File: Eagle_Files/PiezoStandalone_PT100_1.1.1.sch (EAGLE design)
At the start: 67 parts, among them J1 CON-MOLEX-4P-1.25MM048, U1 ATMEGA48PA-MMHR28M1-L, U2 L78L05ACU, U3 LM2902QT

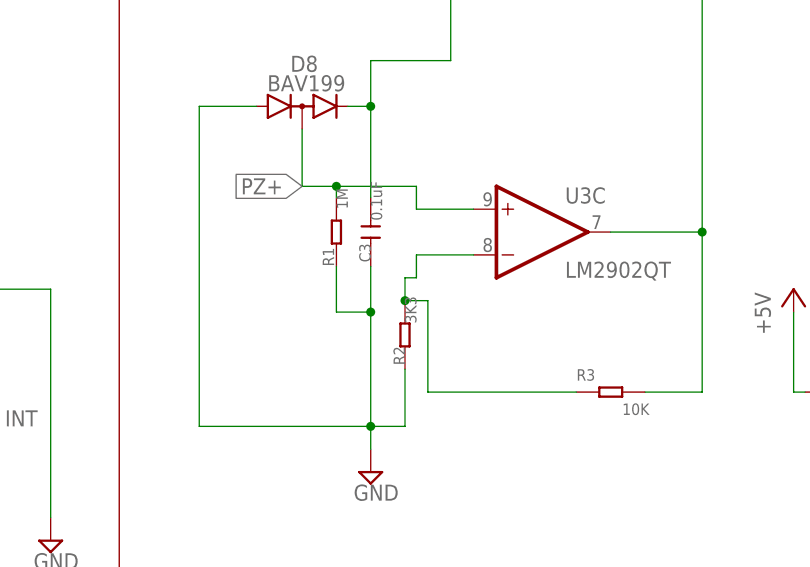
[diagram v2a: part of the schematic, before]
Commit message: Pushing changed files saved after exporting gerber
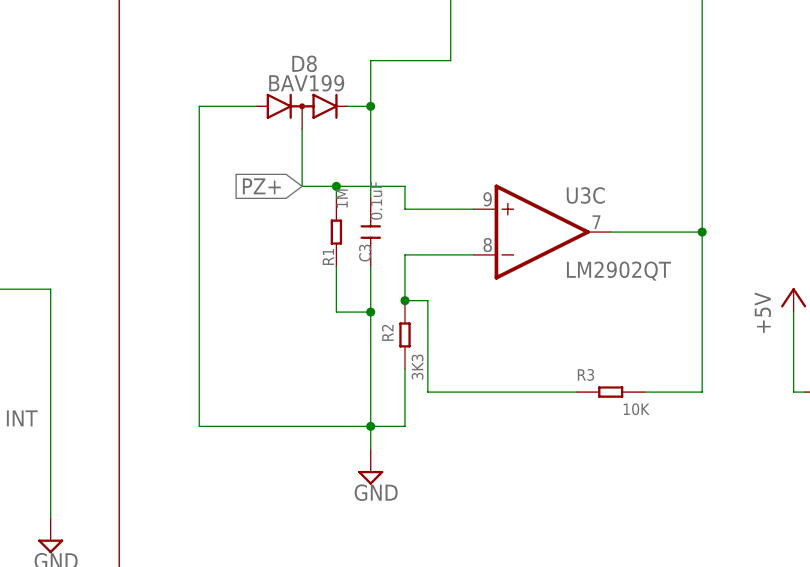
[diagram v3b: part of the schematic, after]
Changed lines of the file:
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@@
 </instance>
 <instance part="R2" gate="G$1" x="203.2" y="195.58" smashed="yes" rot="R90">
-<attribute name="NAME" x="201.93" y="194.31" size="1.27" layer="95" ratio="10" rot="R270"/>
-<attribute name="VALUE" x="204.47" y="196.85" size="1.27" layer="96" ratio="10" rot="R90"/>
+<attribute name="NAME" x="200.66" y="196.85" size="1.27" layer="95" ratio="10" rot="R270"/>
+<attribute name="VALUE" x="205.232" y="190.5" size="1.27" layer="96" ratio="10" rot="R90"/>
 </instance>
 <instance part="R10" gate="G$1" x="251.46" y="189.23" smashed="yes" rot="R180">
@@
 <pinref part="D8" gate="G$1" pin="AC"/>
 <wire x1="191.77" y1="218.44" x2="191.77" y2="212.09" width="0.1524" layer="91"/>
-<wire x1="204.47" y1="212.09" x2="195.58" y2="212.09" width="0.1524" layer="91"/>
+<wire x1="203.2" y1="212.09" x2="195.58" y2="212.09" width="0.1524" layer="91"/>
 <pinref part="R1" gate="G$1" pin="2"/>
 <wire x1="195.58" y1="212.09" x2="195.58" y2="210.82" width="0.1524" layer="91"/>
 <wire x1="195.58" y1="212.09" x2="191.77" y2="212.09" width="0.1524" layer="91"/>
 <junction x="195.58" y="212.09"/>
-<wire x1="204.47" y1="209.55" x2="204.47" y2="212.09" width="0.1524" layer="91"/>
+<wire x1="203.2" y1="209.55" x2="203.2" y2="212.09" width="0.1524" layer="91"/>
 <pinref part="U3" gate="C" pin="+IN"/>
-<wire x1="210.82" y1="209.55" x2="204.47" y2="209.55" width="0.1524" layer="91"/>
+<wire x1="210.82" y1="209.55" x2="203.2" y2="209.55" width="0.1524" layer="91"/>
 <label x="191.77" y="212.09" size="1.778" layer="95" rot="R180" xref="yes"/>
 </segment>
@@
 <segment>
 <pinref part="R2" gate="G$1" pin="2"/>
-<wire x1="204.47" y1="201.93" x2="203.2" y2="201.93" width="0.1524" layer="91"/>
-<wire x1="203.2" y1="201.93" x2="203.2" y2="199.39" width="0.1524" layer="91"/>
 <wire x1="203.2" y1="199.39" x2="205.74" y2="199.39" width="0.1524" layer="91"/>
 <junction x="203.2" y="199.39"/>
@@
 <wire x1="205.74" y1="199.39" x2="205.74" y2="189.23" width="0.1524" layer="91"/>
 <wire x1="205.74" y1="189.23" x2="222.25" y2="189.23" width="0.1524" layer="91"/>
-<wire x1="204.47" y1="204.47" x2="204.47" y2="201.93" width="0.1524" layer="91"/>
+<wire x1="203.2" y1="204.47" x2="203.2" y2="199.39" width="0.1524" layer="91"/>
 <pinref part="U3" gate="C" pin="-IN"/>
-<wire x1="210.82" y1="204.47" x2="204.47" y2="204.47" width="0.1524" layer="91"/>
-</segment>
-</net>
+<wire x1="210.82" y1="204.47" x2="203.2" y2="204.47" width="0.1524" layer="91"/>
+</segment>
+</net>
